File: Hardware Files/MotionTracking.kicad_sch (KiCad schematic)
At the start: 22 parts, among them J1 Micro_SD_Card_Det1, J2 USB_B_Micro, U1 LSM6DSV16XTR, U2 ADP2302ARDZ-3.3, U4 STM32F411RET6, Y1 16MHz

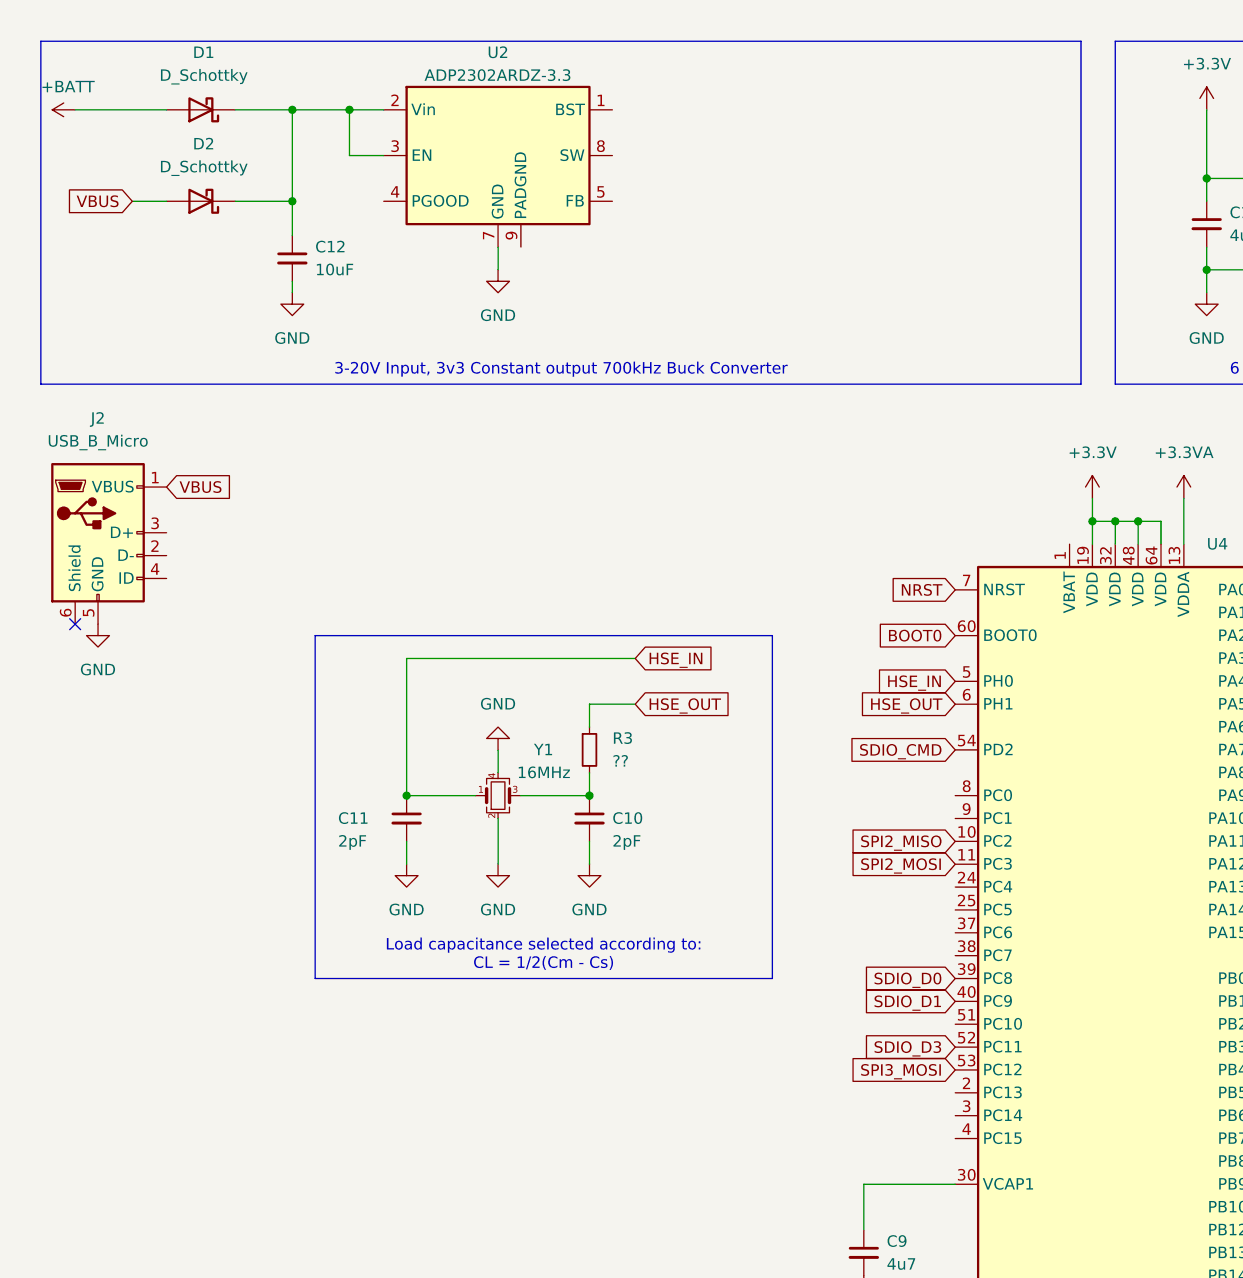
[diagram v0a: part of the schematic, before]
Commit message: Other buck converter changes? or just an autosave?
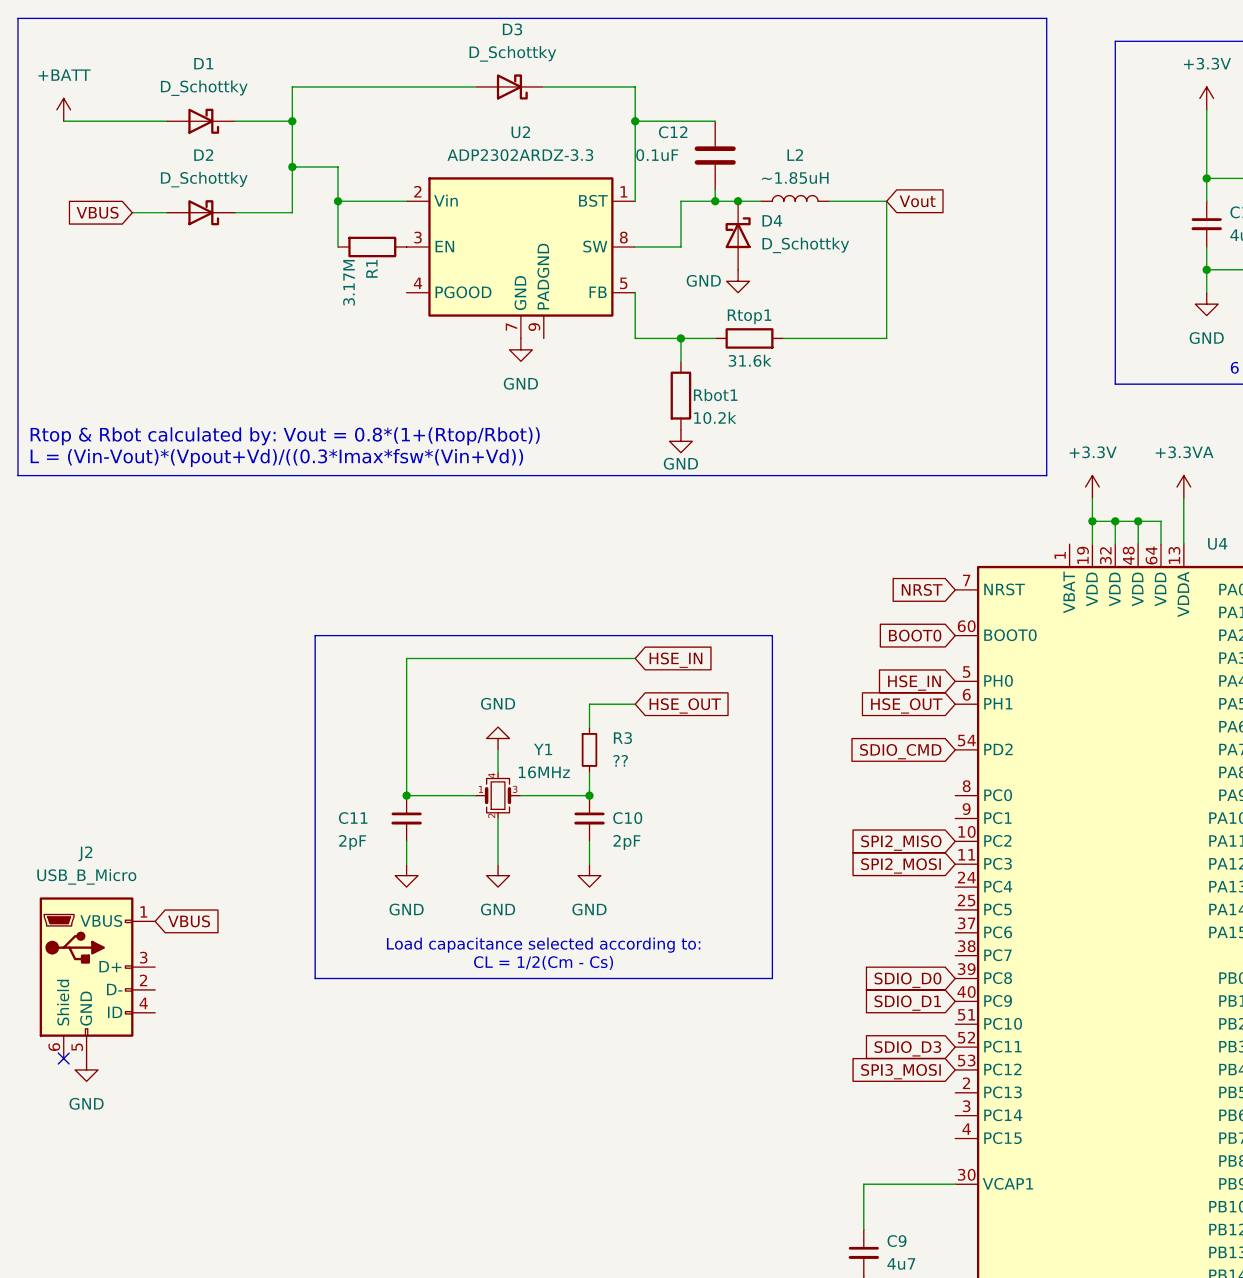
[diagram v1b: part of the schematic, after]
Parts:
- removed C12: 10uF, symbol Device:C_Small
- added C12: 0.1uF, symbol Device:C
- added D3, D4: D_Schottky, symbol Device:D_Schottky
- added L2: ~1.85uH, symbol Device:L
- added R1: 3.17M, symbol Device:R
- added Rbot1: 10.2k, symbol Device:R
- added Rtop1: 31.6k, symbol Device:R
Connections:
- net GND: now also D4.2 (A), Rbot1.2
- net at D1.1 (K), D2.1 (K), U2.2 (Vin): now also D3.2 (A), R1.2; no longer U2.3 (EN)
- net at U2.1 (BST): now also C12.1, D3.1 (K)
- net at U2.5 (FB): now also Rbot1.1, Rtop1.1
- net at U2.8 (SW): now also C12.2, D4.1 (K), L2.1
- new net: R1.1, U2.3 (EN)
- new net Vout: L2.2, Rtop1.2
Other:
- moved on the sheet: J2
